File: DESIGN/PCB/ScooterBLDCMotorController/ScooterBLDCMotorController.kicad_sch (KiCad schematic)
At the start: 32 parts, among them J1 M1 OUTPUT, J10 RC_ENABLE, J11 TO M2 ENCODER, J12 M2 INPUT, J2 TO M1 ENCODER, J3 M1 INPUT, J4 M2 OUTPUT, J5 I2C, J6 TEST SWITCH, J7 RC CH 1, J8 RC CH 2, J9 RC_PWR, U1 , U10 , U2 SN74HC14NR, U3 , U4 Teensy4.0, U5 SN74HC14NR, U6 , U7 5V_Voltage_Regulator, U8 3.3V_Voltage_Regulator, U9 

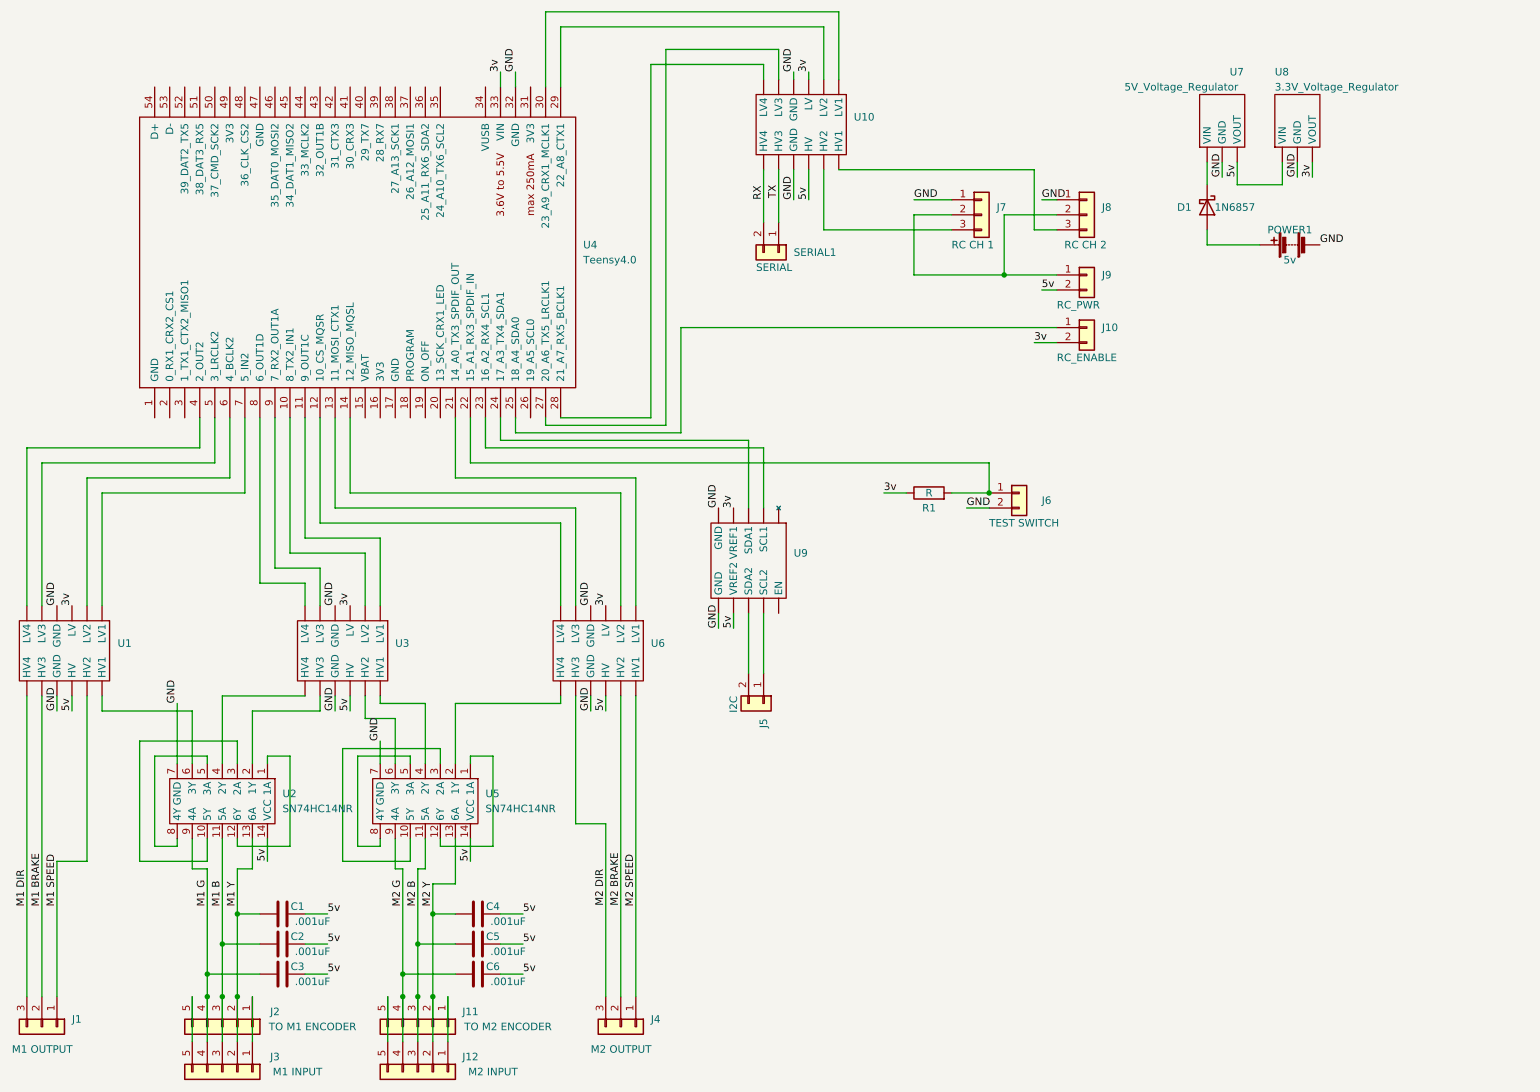
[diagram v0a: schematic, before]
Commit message: Revision 1.2 of MotorController board
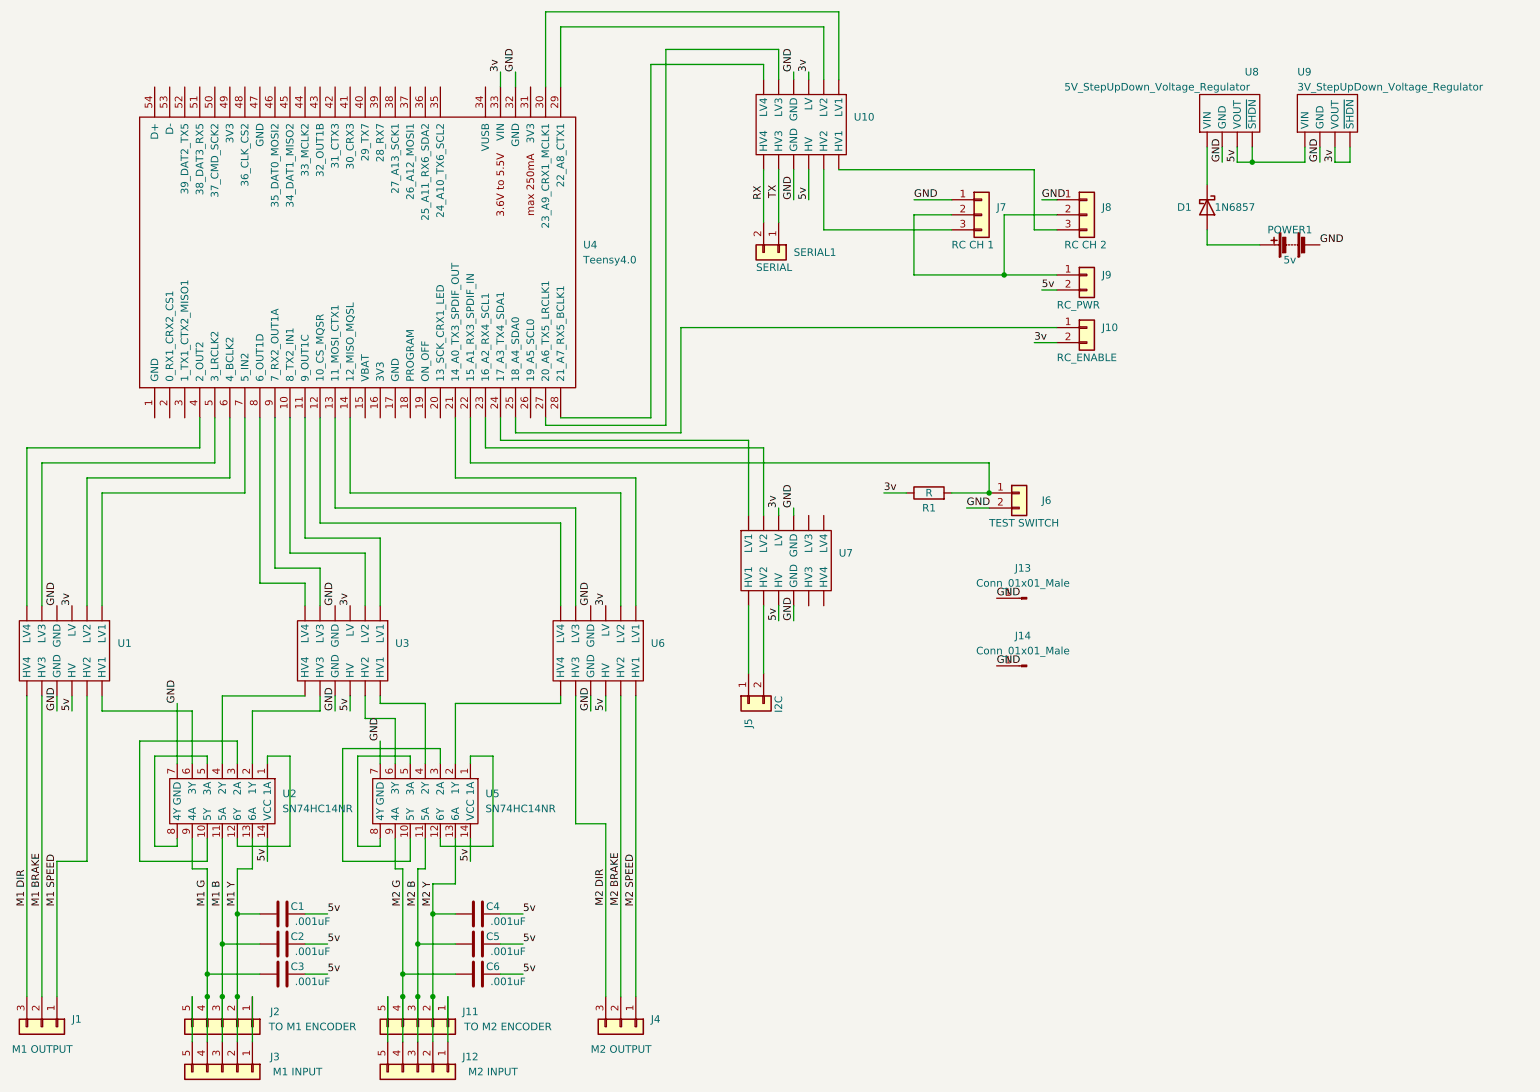
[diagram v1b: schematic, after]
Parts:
- removed U7: 5V_Voltage_Regulator, Custom:Voltage Regulator, symbol Custom:5V_Voltage_Regulator
- removed U8: 3.3V_Voltage_Regulator, Custom:Voltage Regulator, symbol Custom:3.3V_Voltage_Regulator
- removed U9: (no value), Custom:I2C Level Shifter, symbol Custom:I2C_Level_Shifter
- added J13, J14: Conn_01x01_Male, Connector_PinHeader_2.54mm:PinHeader_1x01_P2.54mm_Vertical, symbol Connector:Conn_01x01_Male
- added U7: (no value), Custom:Level Shifter, symbol Custom:Level_Shifter
- added U8: 5V_StepUpDown_Voltage_Regulator, Custom:StepUpDown Voltage Regulator, symbol Custom:5V_StepUpDown_Voltage_Regulator
- added U9: 3V_StepUpDown_Voltage_Regulator, Custom:StepUpDown Voltage Regulator, symbol Custom:3V_StepUpDown_Voltage_Regulator
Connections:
- net 3v: now also U7.9 (LV), U9.3 (VOUT), U9.4 (~{SHDN})
- net 5v: now also U7.4 (HV), U8.3 (VOUT), U8.4 (~{SHDN}), U9.1 (VIN)
- net GND: now also J13.1 (Pin_1), J14.1 (Pin_1), U7.10 (GND), U7.3 (GND), U8.2 (GND), U9.2 (GND)
- net at D1.1 (K): now also U8.1 (VIN)
- net at J5.1 (Pin_1): now also U7.6 (HV1)
- net at J5.2 (Pin_2): now also U7.5 (HV2)
- net at U4.23 (16_A2_RX4_SCL1): now also U7.8 (LV2)
- net at U4.24 (17_A3_TX4_SDA1): now also U7.7 (LV1)
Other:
- moved on the sheet: J5
